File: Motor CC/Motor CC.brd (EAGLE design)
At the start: 58.4 x 100 mm, 11 parts, among them IC1 L298

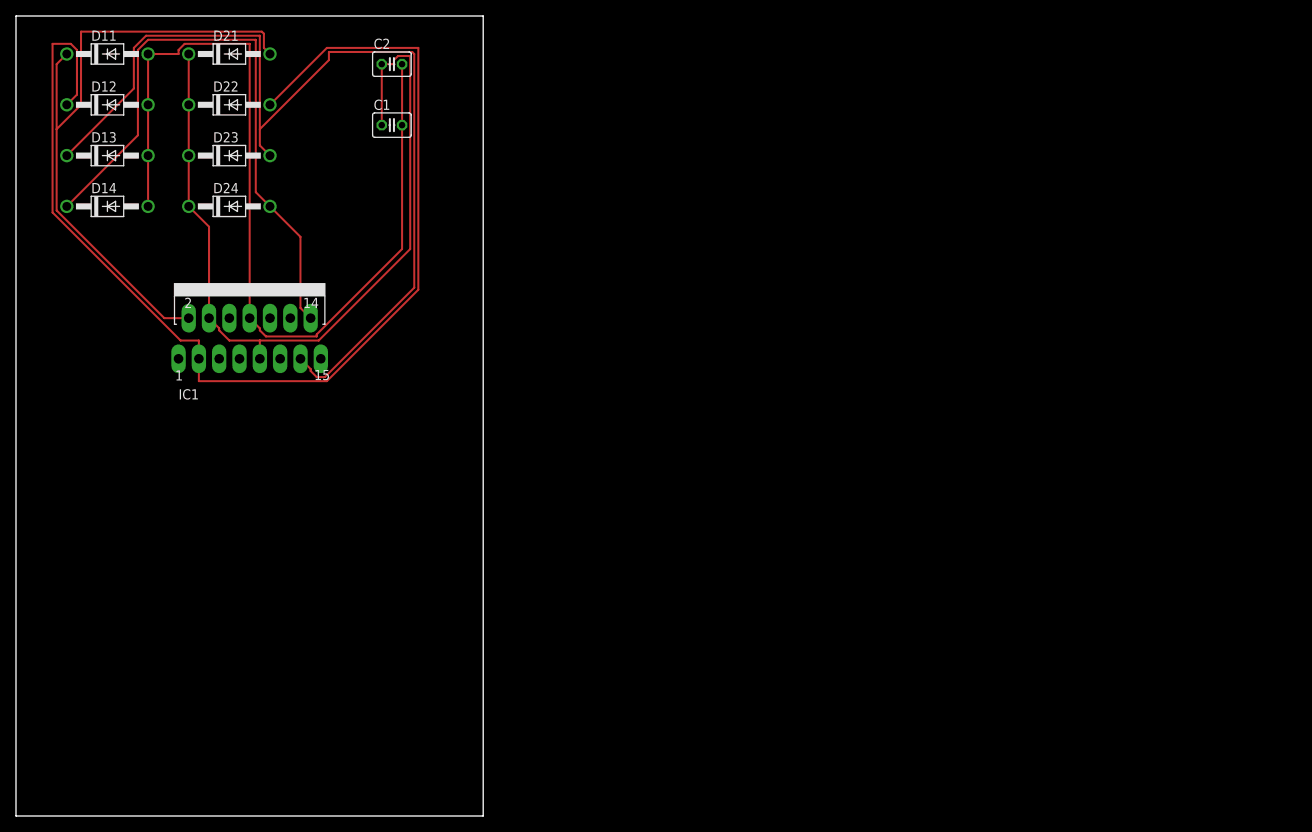
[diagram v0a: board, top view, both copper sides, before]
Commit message: Motors DC finished :D
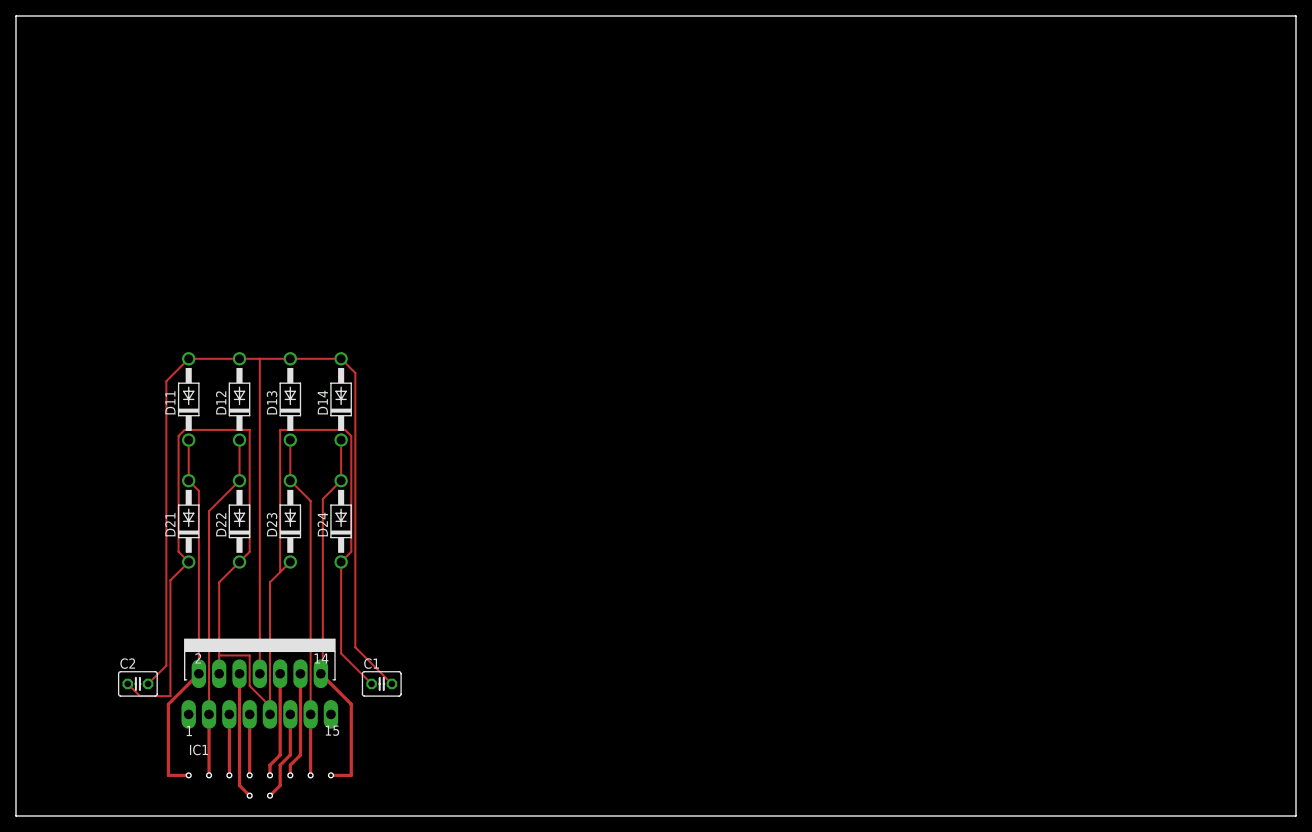
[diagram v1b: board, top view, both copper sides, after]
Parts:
- moved C2 83.7 mm to (15.2, 16.5)
- moved C1 69.9 mm to (45.7, 16.5)
- moved D21 58.6 mm to (21.6, 36.8), turned to 90 degrees
- moved D22 52.1 mm to (27.9, 36.8), turned to 90 degrees
- moved D23 46.4 mm to (34.3, 36.8), turned to 90 degrees
- moved IC1 44.5 mm to (30.5, 20.3)
- moved D11 44.4 mm to (21.6, 52.1), turned to 90 degrees
- moved D24 41.8 mm to (40.6, 36.8), turned to 90 degrees
- moved D12 40.4 mm to (27.9, 52.1), turned to 90 degrees
- moved D13 38.1 mm to (34.3, 52.1), turned to 90 degrees
- moved D14 37.9 mm to (40.6, 52.1), turned to 90 degrees
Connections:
- new net N$10: IC1.12
- new net N$5: IC1.6
- new net N$6: IC1.11
- new net N$7: IC1.5
- new net N$8: IC1.7
- new net N$9: IC1.10
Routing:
- net N$3: track 145.7 -> 43.5 mm
- net N$4: track 122.0 -> 43.0 mm
- net VSS: track 103.6 -> 172.6 mm
- net N$2: track 81.4 -> 46.6 mm
- net GND: track 114.8 -> 144.4 mm
- net N$1: track 76.1 -> 47.2 mm
- net N$5: track 0.00 -> 15.8 mm
- net N$9: track 0.00 -> 13.2 mm
- net N$10: track 0.00 -> 13.2 mm
- net N$6: track 0.00 -> 11.2 mm
- net N$8: track 0.00 -> 7.62 mm
- net N$7: track 0.00 -> 7.62 mm
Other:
- board size 58.4 x 100 mm -> 160 x 100 mm
